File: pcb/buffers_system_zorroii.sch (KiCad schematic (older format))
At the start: 39 parts, among them U5 74LVCH162245A

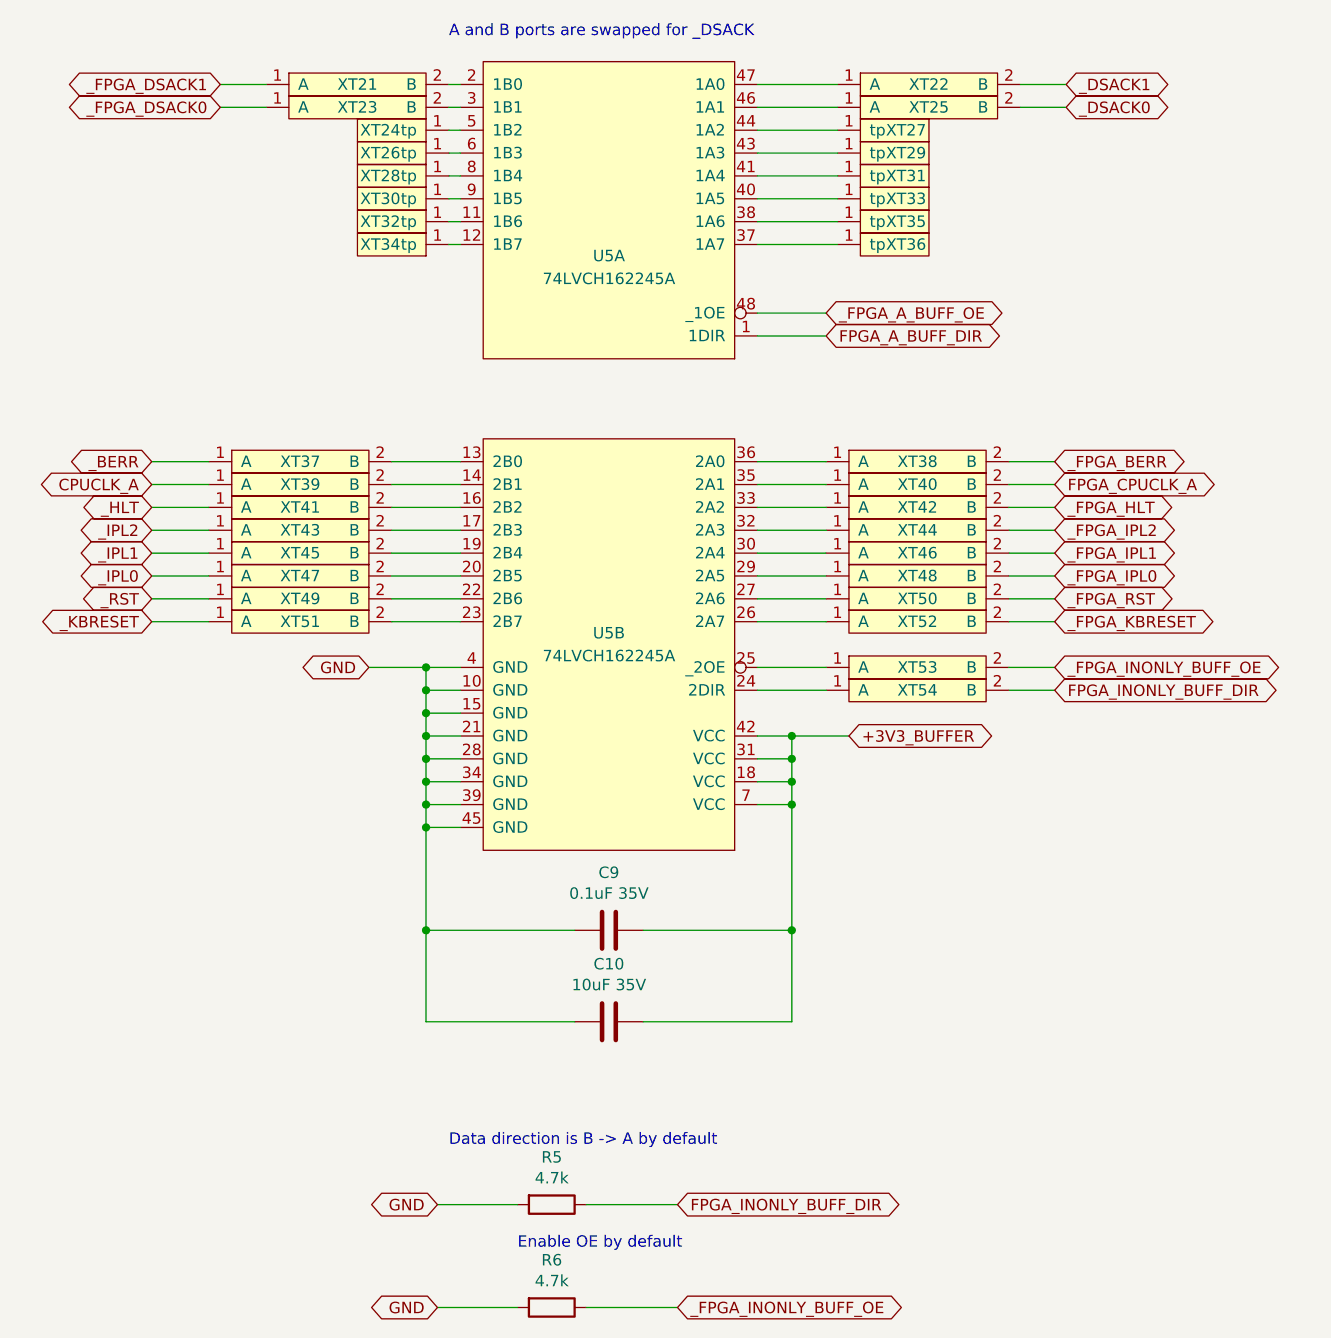
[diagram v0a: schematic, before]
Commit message: working on pcb 2
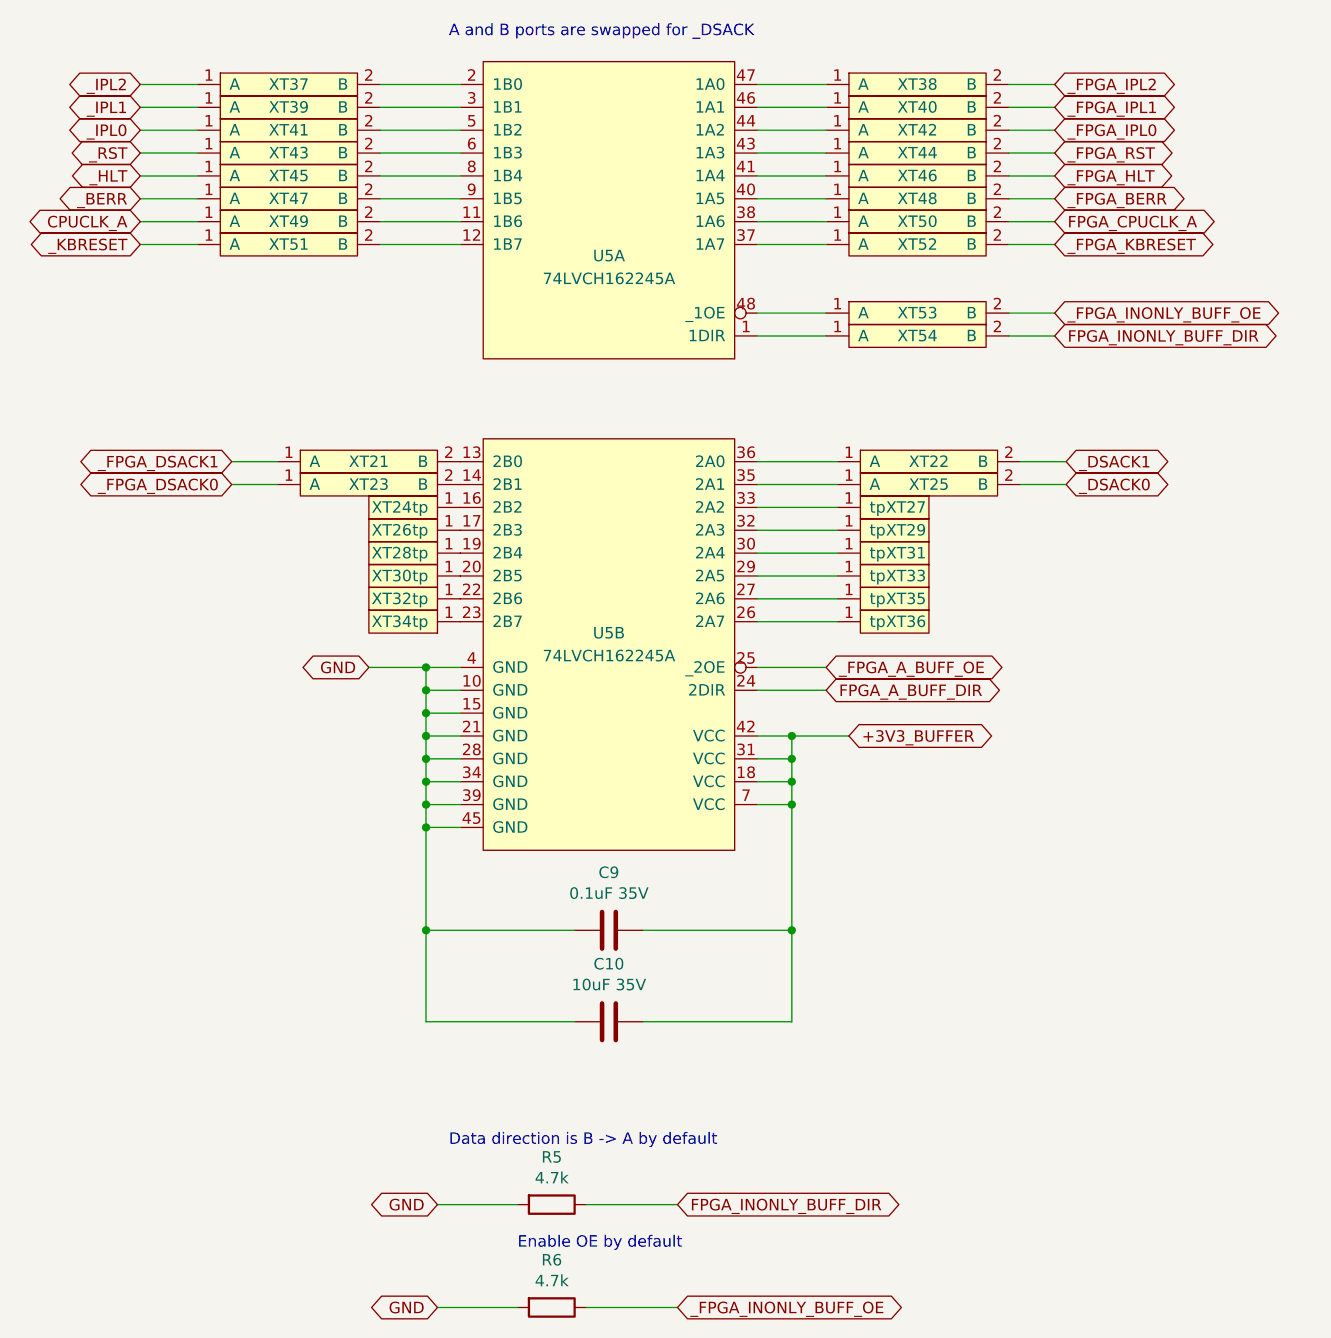
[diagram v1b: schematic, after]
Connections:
- net CPUCLK_A: now also XT49.1 (A); no longer XT39.1 (A)
- net FPGA_A_BUFF_DIR: now also U5.24 (2DIR); no longer U5.1 (1DIR)
- net FPGA_CPUCLK_A: now also XT50.2 (B); no longer XT40.2 (B)
- net _BERR: now also XT47.1 (A); no longer XT37.1 (A)
- net _FPGA_A_BUFF_OE: now also U5.25 (_2OE); no longer U5.48 (_1OE)
- net _FPGA_BERR: now also XT48.2 (B); no longer XT38.2 (B)
- net _FPGA_HLT: now also XT46.2 (B); no longer XT42.2 (B)
- net _FPGA_IPL0: now also XT42.2 (B); no longer XT48.2 (B)
- net _FPGA_IPL1: now also XT40.2 (B); no longer XT46.2 (B)
- net _FPGA_IPL2: now also XT38.2 (B); no longer XT44.2 (B)
- net _FPGA_RST: now also XT44.2 (B); no longer XT50.2 (B)
- net _HLT: now also XT45.1 (A); no longer XT41.1 (A)
- net _IPL0: now also XT41.1 (A); no longer XT47.1 (A)
- net _IPL1: now also XT39.1 (A); no longer XT45.1 (A)
- net _IPL2: now also XT37.1 (A); no longer XT43.1 (A)
- net _RST: now also XT43.1 (A); no longer XT49.1 (A)
- net at XT21.2 (B): now also U5.13 (2B0); no longer U5.2 (1B0)
- net at XT23.2 (B): now also U5.14 (2B1); no longer U5.3 (1B1)
- net at XT37.2 (B): now also U5.2 (1B0); no longer U5.13 (2B0)
- net at XT39.2 (B): now also U5.3 (1B1); no longer U5.14 (2B1)
- net at XT41.2 (B): now also U5.5 (1B2); no longer U5.16 (2B2)
- net at XT43.2 (B): now also U5.6 (1B3); no longer U5.17 (2B3)
- net at XT45.2 (B): now also U5.8 (1B4); no longer U5.19 (2B4)
- net at XT47.2 (B): now also U5.9 (1B5); no longer U5.20 (2B5)
- net at XT49.2 (B): now also U5.11 (1B6); no longer U5.22 (2B6)
- net at XT51.2 (B): now also U5.12 (1B7); no longer U5.23 (2B7)
- net at XT32.1 (tp): now also U5.22 (2B6); no longer U5.11 (1B6)
- net at XT34.1 (tp): now also U5.23 (2B7); no longer U5.12 (1B7)
- net at U5.37 (1A7): now also XT52.1 (A); no longer XT36.1 (tp)
- net at U5.38 (1A6): now also XT50.1 (A); no longer XT35.1 (tp)
- net at U5.40 (1A5): now also XT48.1 (A); no longer XT33.1 (tp)
- net at U5.41 (1A4): now also XT46.1 (A); no longer XT31.1 (tp)
- net at U5.43 (1A3): now also XT44.1 (A); no longer XT29.1 (tp)
- net at U5.44 (1A2): now also XT42.1 (A); no longer XT27.1 (tp)
- net at U5.46 (1A1): now also XT40.1 (A); no longer XT25.1 (A)
- net at U5.47 (1A0): now also XT38.1 (A); no longer XT22.1 (A)
- net at XT24.1 (tp): now also U5.16 (2B2); no longer U5.5 (1B2)
- net at XT26.1 (tp): now also U5.17 (2B3); no longer U5.6 (1B3)
- net at XT28.1 (tp): now also U5.19 (2B4); no longer U5.8 (1B4)
- net at XT30.1 (tp): now also U5.20 (2B5); no longer U5.9 (1B5)
- net at XT54.1 (A): now also U5.1 (1DIR); no longer U5.24 (2DIR)
- net at XT53.1 (A): now also U5.48 (_1OE); no longer U5.25 (_2OE)
- net at U5.26 (2A7): now also XT36.1 (tp); no longer XT52.1 (A)
- net at U5.27 (2A6): now also XT35.1 (tp); no longer XT50.1 (A)
- net at U5.29 (2A5): now also XT33.1 (tp); no longer XT48.1 (A)
- net at U5.30 (2A4): now also XT31.1 (tp); no longer XT46.1 (A)
- net at U5.32 (2A3): now also XT29.1 (tp); no longer XT44.1 (A)
- net at U5.33 (2A2): now also XT27.1 (tp); no longer XT42.1 (A)
- net at U5.35 (2A1): now also XT25.1 (A); no longer XT40.1 (A)
- net at U5.36 (2A0): now also XT22.1 (A); no longer XT38.1 (A)
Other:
- moved on the sheet: XT21, XT22, XT23, XT24, XT25, XT26, XT27, XT28, XT29, XT30, XT31, XT32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

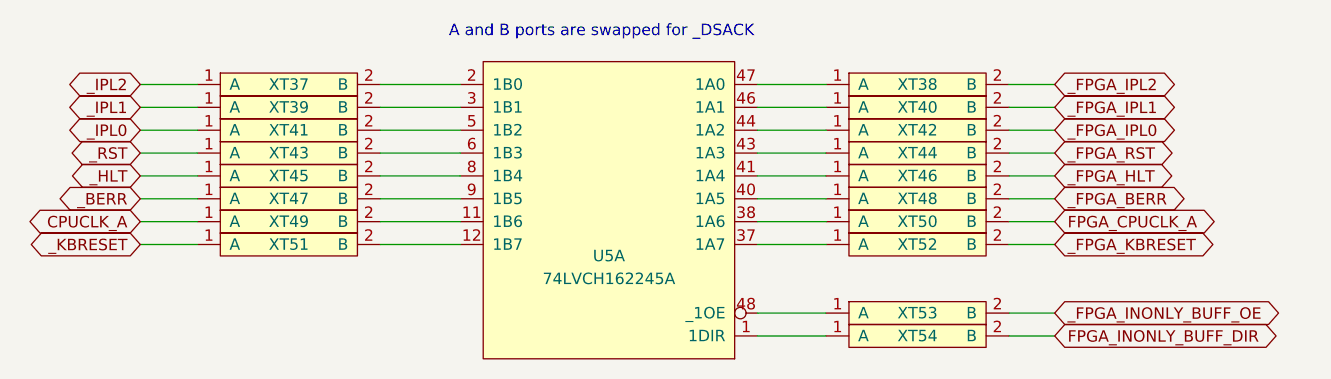
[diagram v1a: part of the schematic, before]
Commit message: working on pcb
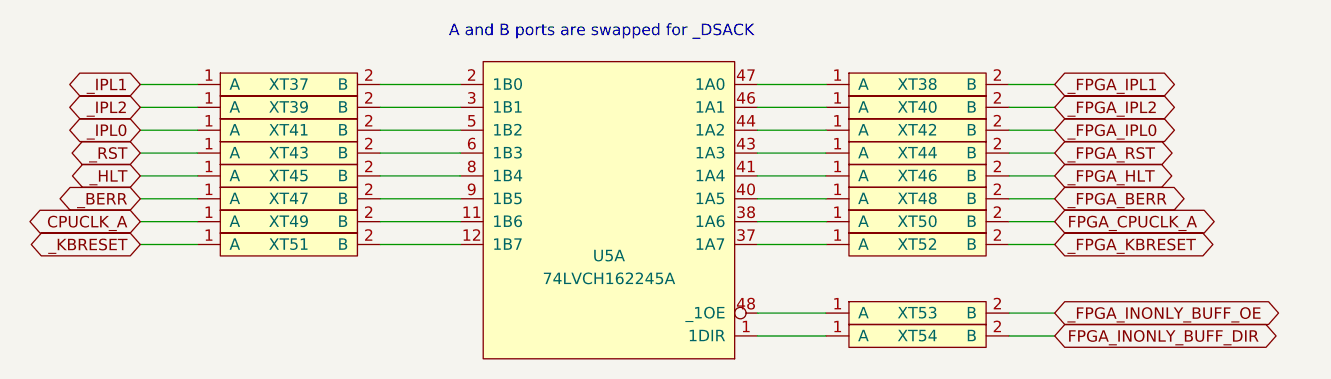
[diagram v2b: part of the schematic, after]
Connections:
- net _FPGA_IPL1: now also XT38.2 (B); no longer XT40.2 (B)
- net _FPGA_IPL2: now also XT40.2 (B); no longer XT38.2 (B)
- net _IPL1: now also XT37.1 (A); no longer XT39.1 (A)
- net _IPL2: now also XT39.1 (A); no longer XT37.1 (A)
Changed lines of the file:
@@
 Text GLabel 2100 1750 0    50   BiDi ~ 0
 _IPL0
+Text GLabel 2100 1550 0    50   BiDi ~ 0
+_IPL1
 Text GLabel 2100 1650 0    50   BiDi ~ 0
-_IPL1
-Text GLabel 2100 1550 0    50   BiDi ~ 0
 _IPL2
 Text GLabel 2100 1850 0    50   BiDi ~ 0
@@
 Text GLabel 6100 1950 2    50   BiDi ~ 0
 _FPGA_HLT
+Text GLabel 6100 1650 2    50   BiDi ~ 0
+_FPGA_IPL2
 Text GLabel 6100 1550 2    50   BiDi ~ 0
-_FPGA_IPL2
-Text GLabel 6100 1650 2    50   BiDi ~ 0
 _FPGA_IPL1
 Text GLabel 6100 1750 2    50   BiDi ~ 0
